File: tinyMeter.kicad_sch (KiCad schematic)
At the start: 93 parts, among them J1 USB_MASTER, J2 DC_POWER, J3 USB_POWER, J4 USBA_OUT_2, J5 USBA_OUT_1, J6 DC_POWER, J7 Debug, J8 External antenna, Q1 100N03A, Q2 100N03A, Q3 100N03A, Q4 SS8050, SW1 SW_Push, SW2 SW_Push, SW3 SW_Push, SW4 SW_Push, SW5 SW_Push, SW6 Boot, SW7 Reset, U1 ESP32-S3, U2 INA219AxD, U3 INA219AxD, U4 INA219AxD, U5 AMS1117-3.3, Y1 Crystal_GND24

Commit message: Working on v2
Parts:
- removed AE1: PCB antenna, Library:ESPRESSIF_ESP32_MIFA_2.4GHz_Right, symbol Device:Antenna_Loop
- removed C1, C2: 10u, Capacitor_SMD:C_0805_2012Metric, symbol Device:C
- removed C10, C11, C16, C17, C19, C20, C21, C22, C23: 100n, Capacitor_SMD:C_0603_1608Metric, symbol Device:C
- removed C12, C15, C18: 1u, Capacitor_SMD:C_0603_1608Metric, symbol Device:C
- removed C13, C14, C3, C6: 10u, Capacitor_SMD:C_0603_1608Metric, symbol Device:C
- removed C4, C5: 10p, Capacitor_SMD:C_0603_1608Metric, symbol Device:C
- removed C7, C8, C9: LNA, Capacitor_SMD:C_0603_1608Metric, symbol Device:C
- removed D1: WS2812B, LED_SMD:LED_WS2812B_PLCC4_5.0x5.0mm_P3.2mm, symbol LED:WS2812B
- removed D2: PWR_LED, LED_SMD:LED_0603_1608Metric, symbol PCM_SL_Devices:LED
- removed DS1: ST77xx, Library:ST77XX, symbol Library:ST77xx
- removed J2: DC_POWER, Connector_BarrelJack:BarrelJack_Horizontal, symbol Connector:Barrel_Jack_MountingPin
- removed J3: USB_POWER, Connector_USB:USB_C_Receptacle_HRO_TYPE-C-31-M-12, symbol Connector:USB_C_Receptacle_USB2.0_16P
- removed J4: USBA_OUT_2, Connector_USB:USB_A_Receptacle_GCT_USB1046, symbol Connector:USB_A
- removed J5: USBA_OUT_1, Connector_USB:USB_A_Receptacle_GCT_USB1046, symbol Connector:USB_A
- removed J7: Debug, Connector_PinSocket_2.54mm:PinSocket_1x04_P2.54mm_Horizontal, symbol Connector_Generic:Conn_01x04
- removed J8: External antenna, Connector_Coaxial:U.FL_Hirose_U.FL-R-SMT-1_Vertical, symbol Connector:Conn_Coaxial
- removed L1, L2: L, Inductor_SMD:L_0603_1608Metric, symbol Device:L
- removed L3: 2n, Inductor_SMD:L_0603_1608Metric, symbol Device:L
- removed Q1, Q2, Q3: 100N03A, Package_TO_SOT_SMD:TO-252-2, symbol Transistor_FET:BUK9832-55A
- removed Q4: SS8050, Package_TO_SOT_SMD:SOT-23, symbol Transistor_BJT:SS8050
- removed R1, R2, R3, R4: 5k1, Resistor_SMD:R_0603_1608Metric, symbol Device:R
- removed R10, R6, R7, R9: 0R, Resistor_SMD:R_0603_1608Metric, symbol Device:R
- removed R11, R5, R8: R025, Resistor_SMD:R_2512_6332Metric, symbol Device:R
- removed R12, R13: 220, Resistor_SMD:R_0603_1608Metric, symbol Device:R
- removed R14, R15, R16, R17, R18, R19, R22, R24, R25, R28, R32, R33, R34: 10k, Resistor_SMD:R_0603_1608Metric, symbol Device:R
- removed R20, R21, R23, R31: 1k, Resistor_SMD:R_0603_1608Metric, symbol Device:R
- removed R26, R27: 2k7, Resistor_SMD:R_0603_1608Metric, symbol Device:R
- removed R29: 60, Resistor_SMD:R_0603_1608Metric, symbol Device:R
- removed R30: 100, Resistor_SMD:R_0603_1608Metric, symbol Device:R
- removed SW6: Boot, Button_Switch_SMD:SW_SPST_B3U-1000P, symbol Switch:SW_Push
- removed SW7: Reset, Button_Switch_SMD:SW_SPST_B3U-1000P, symbol Switch:SW_Push
- removed U1: ESP32-S3, Package_DFN_QFN:QFN-56-1EP_7x7mm_P0.4mm_EP4x4mm, symbol MCU_Espressif:ESP32-S3
- removed U2, U3, U4: INA219AxD, Package_SO:SOIC-8_3.9x4.9mm_P1.27mm, symbol Sensor_Energy:INA219AxD
- removed U5: AMS1117-3.3, Package_TO_SOT_SMD:SOT-223-3_TabPin2, symbol Regulator_Linear:AMS1117-3.3
- removed Y1: Crystal_GND24, Library:OSC_XRCGB40M000F4M00R0, symbol Device:Crystal_GND24
- added C1, C2, C7: 10u, Capacitor_SMD:C_0603_1608Metric, symbol TheEvilRoot:C_0603
- added C3: 1u, Capacitor_SMD:C_0603_1608Metric, symbol TheEvilRoot:C_0603
- added C4, C5, C6: 100n, Capacitor_SMD:C_0603_1608Metric, symbol TheEvilRoot:C_0603
- added J10, J2: USB_IN, TheEvilRoot:USB_C_Receptacle_HRO_TYPE-C-31-M-12, symbol TheEvilRoot:USB_C_Receptacle_USB2.0_16P
- added J11: Debug, Connector_PinHeader_1.27mm:PinHeader_1x06_P1.27mm_Vertical, symbol Connector_Generic:Conn_01x06
- added J3: USB_OUT, TheEvilRoot:USB_C_Receptacle_HRO_TYPE-C-31-M-12, symbol TheEvilRoot:USB_C_Receptacle_USB2.0_16P
- added J4: OLED, Connector_PinSocket_2.54mm:PinSocket_1x04_P2.54mm_Vertical, symbol Connector_Generic:Conn_01x04
- added J5: DC_IN, Connector_BarrelJack:BarrelJack_Horizontal, symbol Connector:Barrel_Jack_MountingPin
- added J7, J8: Conn_01x02, TheEvilRoot:SolderWire-SMD-2pin-2.54mm-D3.0, symbol Connector_Generic:Conn_01x02
- added J9: USB_OUT, TheEvilRoot:TE_292303-1, symbol TheEvilRoot:USB_A_TE_292303-1
- added R1, R4, R5: R100, Resistor_SMD:R_2512_6332Metric, symbol TheEvilRoot:R_2512
- added R10, R11, R12, R13, R6, R7, R8, R9: 10k, Resistor_SMD:R_0603_1608Metric, symbol TheEvilRoot:R_0603
- added R14, R15, R2, R3: 5k1, Resistor_SMD:R_0603_1608Metric, symbol TheEvilRoot:R_0603
- added R16, R17, R18, R19, R20: R, Resistor_SMD:R_0603_1608Metric, symbol TheEvilRoot:R_0603
- added R21, R22: 2k7, Resistor_SMD:R_0603_1608Metric, symbol TheEvilRoot:R_0603
- added U1: AP2112K-3.3, Package_TO_SOT_SMD:SOT-23-5, symbol Regulator_Linear:AP2112K-3.3
- added U2: INA3221AIRGVR, TheEvilRoot:QFN65P400X400X100-17N, symbol TheEvilRoot:INA3221AIRGVR
- added U3: ESP32-S3-WROOM-1, TheEvilRoot:ESP32-S3-WROOM-1, symbol TheEvilRoot:ESP32-S3-WROOM-1
- J1: value USB_MASTER -> USB_C_Receptacle_USB2.0_16P; footprint Connector_USB:USB_C_Receptacle_HRO_TYPE-C-31-M-12 -> TheEvilRoot:USB_C_Receptacle_HRO_TYPE-C-31-M-12; symbol Connector:USB_C_Receptacle_USB2.0_16P -> TheEvilRoot:USB_C_Receptacle_USB2.0_16P
- J6: value DC_POWER -> DC_OUT
- SW1: value SW_Push -> A1; footprint Button_Switch_SMD:SW_SPST_B3U-1000P -> TheEvilRoot:IT-1185AP
- SW2: value SW_Push -> A2; footprint Button_Switch_SMD:SW_SPST_B3U-1000P -> TheEvilRoot:IT-1185AP
- SW3: value SW_Push -> A3; footprint Button_Switch_SMD:SW_SPST_B3U-1000P -> TheEvilRoot:IT-1185AP
- SW4: value SW_Push -> A4; footprint Button_Switch_SMD:SW_SPST_B3U-1000P -> TheEvilRoot:IT-1185AP
- SW5: value SW_Push -> A0; footprint Button_Switch_SMD:SW_SPST_B3U-1000P -> TheEvilRoot:IT-1185AP
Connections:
- net DC_POWER_GND is gone; now on net GND: J6.2
- net KEYPAD_K1 is gone; now on net +3V3: SW1.1
- net KEYPAD_K2 is gone; now on net +3V3: SW2.1
- net KEYPAD_K3 is gone; now on net +3V3: SW3.1
- net KEYPAD_K4 is gone; now on net +3V3: SW4.1
- net KEYPAD_K5 is gone; now on net +3V3: SW5.1
- net +3V3: now also C2.1, C3.1, C4.1, C5.1, C6.1, J11.1 (Pin_1), J4.2 (Pin_2), R10.1, R11.1, R12.1, R13.1, R21.1, R22.1, R6.1, R7.1, R8.1, R9.1, U1.5 (VOUT), U2.16 (VPU), U2.4 (VS), U3.2 (3V3)
- net ESP_EN: now also C7.1, J11.4 (Pin_4), R13.2, U3.3 (EN)
- net ESP_RX: now also J11.3 (Pin_3), U3.36 (RXD0)
- net ESP_TX: now also J11.2 (Pin_2), U3.37 (TXD0)
- net GND: now also C1.2, C2.2, C3.2, C4.2, C5.2, C6.2, C7.2, J10.A1 (GND), J10.A12 (GND), J10.B1 (GND), J10.B12 (GND), J11.6 (Pin_6), J2.A1 (GND), J2.A12 (GND), J2.B1 (GND), J2.B12 (GND), J3.A1 (GND), J3.A12 (GND), J3.B1 (GND), J3.B12 (GND), J4.1 (Pin_1), J5.2, J7.1 (Pin_1), J8.1 (Pin_1), J9.4 (GND), R14.2, R15.2, R2.2, R3.2, U1.2 (GND), U2.17 (EXP), U2.3 (GND), U2.5 (A0), U3.1 (GND), U3.40 (GND), U3.41 (GND)
- net METER_SCL: now also R10.2, U2.6 (SCL), U3.35 (IO42)
- net METER_SDA: now also R11.2, U2.7 (SDA), U3.34 (IO41)
- net USB_MASTER_CC1: now also R3.1
- net USB_MASTER_CC2: now also R2.1
- net USB_MASTER_D+: now also U3.14 (USB_D+)
- net USB_MASTER_D-: now also U3.13 (USB_D-)
- net at SW2.2: now also R17.1
- net at SW3.2: now also R18.1
- net at SW4.2: now also R19.1
- net at SW1.2: now also R16.1
- net at SW5.2: now also R20.1
- net DC_POWER_VCC renamed METER_3-
- net METER_3-: now also R4.2, U2.1 (IN-3)
- net USB_VBUS renamed VBUS
- net VBUS: now also C1.1, U1.1 (VIN), U1.3 (EN)
- new net ESP_BOOT: J11.5 (Pin_5), R12.2, U3.27 (IO0)
- new net METER_1+: J2.A4 (VBUS), J2.A9 (VBUS), J2.B4 (VBUS), J2.B9 (VBUS), J7.2 (Pin_2), R1.1, U2.12 (IN+1)
- new net METER_1-: J3.A4 (VBUS), J3.A9 (VBUS), J3.B4 (VBUS), J3.B9 (VBUS), J8.2 (Pin_2), R1.2, U2.11 (IN-1)
- new net METER_2+: J10.A4 (VBUS), J10.A9 (VBUS), J10.B4 (VBUS), J10.B9 (VBUS), R5.1, U2.15 (IN+2)
- new net METER_2-: J9.1 (VBUS), R5.2, U2.14 (IN-2)
- new net METER_3+: J5.1, R4.1, U2.2 (IN+3)
- new net METER_CRIT: R6.2, U2.9 (CRITICAL), U3.32 (IO39)
- new net METER_TIMING: R8.2, U2.13 (TC), U3.26 (IO45)
- new net METER_VALID: R7.2, U2.10 (PV), U3.31 (IO38)
- new net METER_WARN: R9.2, U2.8 (WARNING), U3.33 (IO40)
- new net OLED_SCL: J4.3 (Pin_3), R22.2, U3.19 (IO11)
- new net OLED_SDA: J4.4 (Pin_4), R21.2, U3.18 (IO10)
- new net SW_A0: R20.2, U3.12 (IO8)
- new net SW_A1: R16.2, U3.11 (IO18)
- new net SW_A2: R17.2, U3.10 (IO17)
- new net SW_A3: R18.2, U3.9 (IO16)
- new net SW_A4: R19.2, U3.8 (IO15)
- new net USB_A_CC1: J10.A5 (CC1), R14.1
- new net USB_A_CC2: J10.B5 (CC2), R15.1
- new net USB_A_D+: J10.A6 (D+), J10.B6 (D+), J9.3 (D+)
- new net USB_A_D-: J10.A7 (D-), J10.B7 (D-), J9.2 (D-)
- new net USB_C_CC1: J2.A5 (CC1), J3.A5 (CC1)
- new net USB_C_CC2: J2.B5 (CC2), J3.B5 (CC2)
- new net USB_C_D1+: J2.B6 (D+), J3.B6 (D+)
- new net USB_C_D1-: J2.A7 (D-), J3.A7 (D-)
- new net USB_C_D2+: J2.A6 (D+), J3.A6 (D+)
- new net USB_C_D2-: J2.B7 (D-), J3.B7 (D-)
- new net USB_C_SBU1: J2.A8 (SBU1), J3.A8 (SBU1)
- new net USB_C_SBU2: J2.B8 (SBU2), J3.B8 (SBU2)
- no-connect marks 39 -> 28
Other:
- note added: "TODO: 1. Test points for - Meter +/- - 3.3V - Meter open-drains params 2. Debug LEDs for MCU 3. LEDs for open-drains meter outputs"

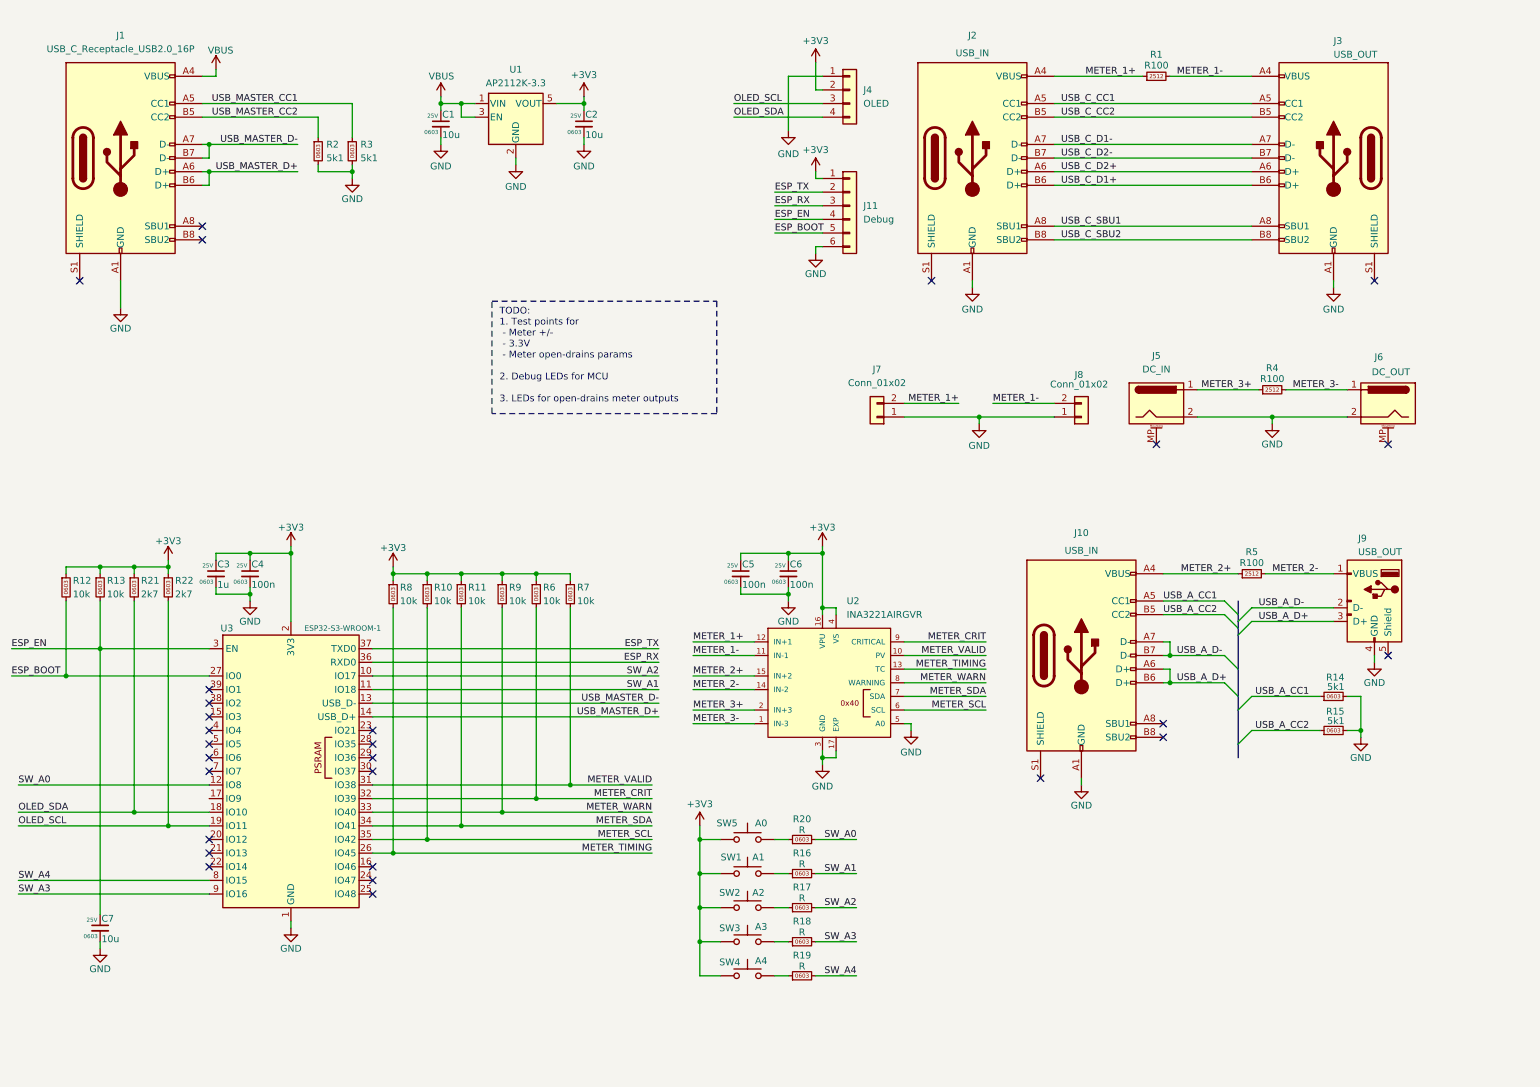
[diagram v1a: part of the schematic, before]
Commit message: Version 2 finish
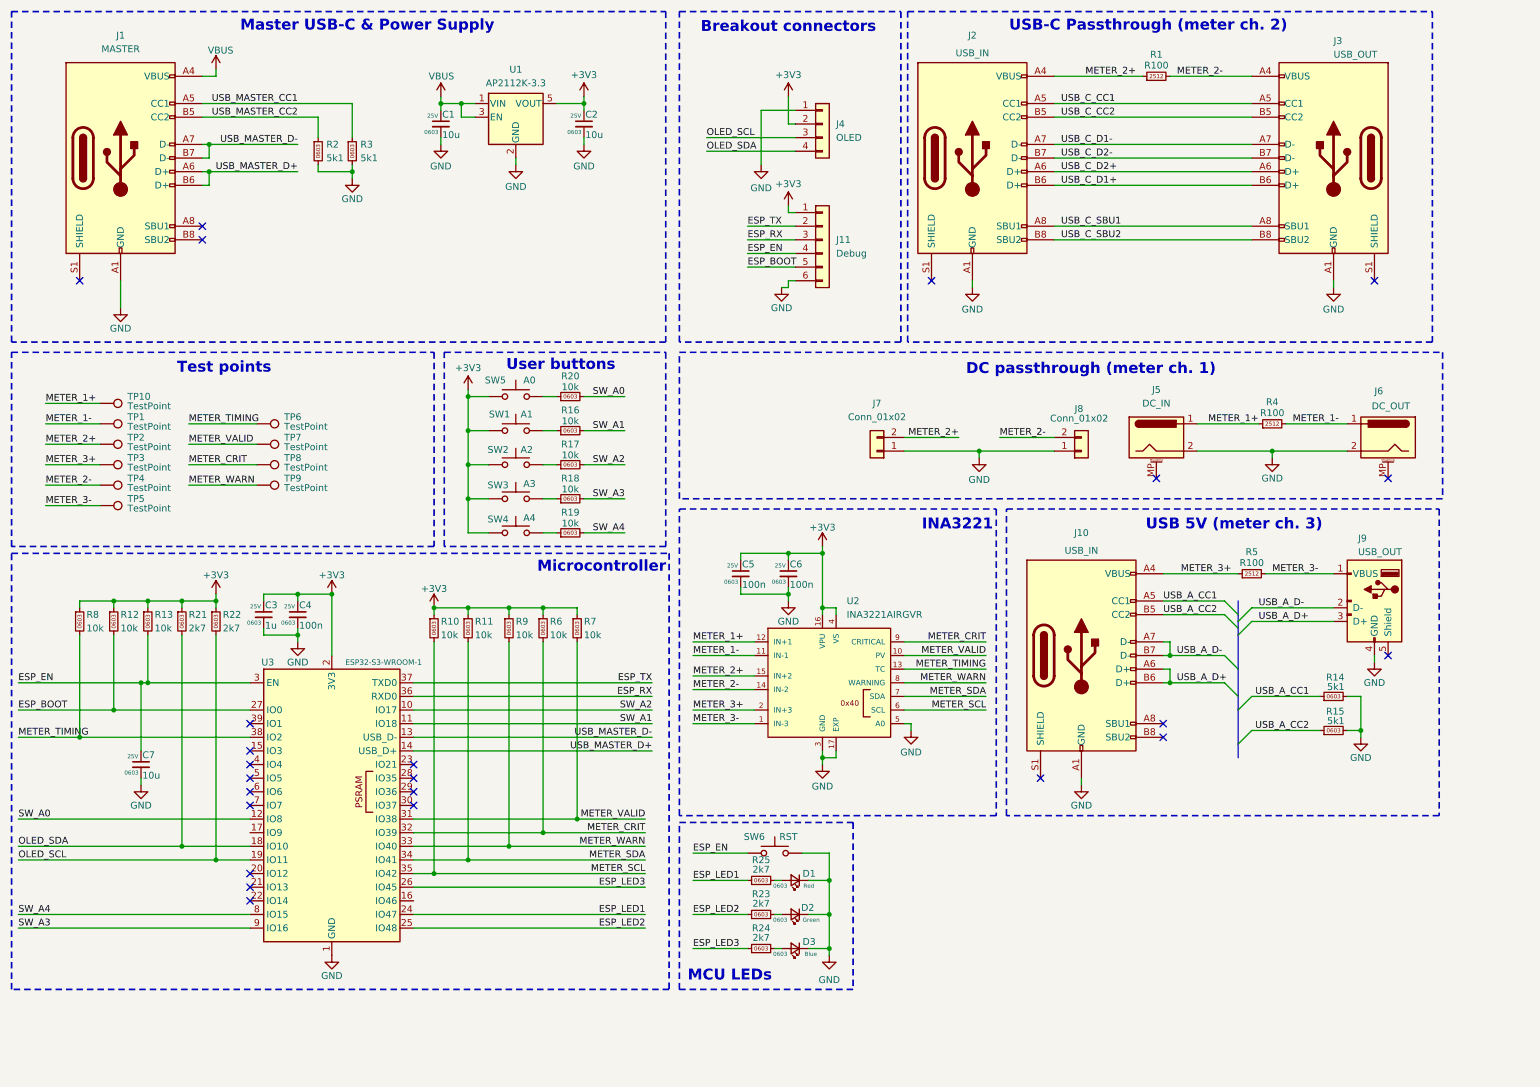
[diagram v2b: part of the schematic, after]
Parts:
- added D1: Red, LED_SMD:LED_0603_1608Metric, symbol TheEvilRoot:LED_0603_Red
- added D2: Green, LED_SMD:LED_0603_1608Metric, symbol TheEvilRoot:LED_0603_Green
- added D3: Blue, LED_SMD:LED_0603_1608Metric, symbol TheEvilRoot:LED_0603_Blue
- added R23, R24, R25: 2k7, Resistor_SMD:R_0603_1608Metric, symbol TheEvilRoot:R_0603
- added SW6: RST, TheEvilRoot:KLS7-TS3401, symbol Switch:SW_Push
- added TP1, TP10, TP2, TP3, TP4, TP5, TP6, TP7, TP8, TP9: TestPoint, TestPoint:TestPoint_Pad_D1.0mm, symbol Connector:TestPoint
- J1: value USB_C_Receptacle_USB2.0_16P -> MASTER
- J7, J8: footprint TheEvilRoot:SolderWire-SMD-2pin-2.54mm-D3.0 -> Connector_PinHeader_2.54mm:PinHeader_1x02_P2.54mm_Vertical
- R16, R17, R18, R19, R20: value R -> 10k
- SW1, SW2, SW3, SW4, SW5: footprint TheEvilRoot:IT-1185AP -> TheEvilRoot:KLS7-TS3401
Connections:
- net ESP_EN: now also SW6.1
- net GND: now also D1.1 (K), D2.1 (K), D3.1 (K), SW6.2
- net METER_1+: now also J5.1, R4.1, TP10.1; no longer J2.A4 (VBUS), J2.A9 (VBUS), J2.B4 (VBUS), J2.B9 (VBUS), J7.2 (Pin_2), R1.1
- net METER_1-: now also J6.1, R4.2, TP1.1; no longer J3.A4 (VBUS), J3.A9 (VBUS), J3.B4 (VBUS), J3.B9 (VBUS), J8.2 (Pin_2), R1.2
- net METER_2+: now also J2.A4 (VBUS), J2.A9 (VBUS), J2.B4 (VBUS), J2.B9 (VBUS), J7.2 (Pin_2), R1.1, TP2.1; no longer J10.A4 (VBUS), J10.A9 (VBUS), J10.B4 (VBUS), J10.B9 (VBUS), R5.1
- net METER_2-: now also J3.A4 (VBUS), J3.A9 (VBUS), J3.B4 (VBUS), J3.B9 (VBUS), J8.2 (Pin_2), R1.2, TP4.1; no longer J9.1 (VBUS), R5.2
- net METER_3+: now also J10.A4 (VBUS), J10.A9 (VBUS), J10.B4 (VBUS), J10.B9 (VBUS), R5.1, TP3.1; no longer J5.1, R4.1
- net METER_3-: now also J9.1 (VBUS), R5.2, TP5.1; no longer J6.1, R4.2
- net METER_CRIT: now also TP8.1
- net METER_TIMING: now also U3.38 (IO2), TP6.1; no longer U3.26 (IO45)
- net METER_VALID: now also TP7.1
- net METER_WARN: now also TP9.1
- net ESP_LED1: now reaches U3.24 (IO47)
- net ESP_LED1: now also R25.1
- net ESP_LED2: now reaches U3.25 (IO48)
- net ESP_LED2: now also R23.1
- new net: D1.2 (A), R25.2
- new net: D2.2 (A), R23.2
- new net: D3.2 (A), R24.2
- new net ESP_LED3: R24.1, U3.26 (IO45)
- no-connect marks 28 -> 24
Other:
- note added: "Breakout connectors"
- note added: "DC passthrough (meter ch. 1)"
- note added: "INA3221"
- note added: "MCU LEDs"
- note added: "Master USB-C & Power Supply"
- note added: "Microcontroller"
- note added: "Test points"
- note added: "USB 5V (meter ch. 3)"
- note added: "USB-C Passthrough (meter ch. 2)"
- note added: "User buttons"
- note removed: "TODO: 1. Test points for - Meter +/- - 3.3V - Meter open-drains params 2. Debug LEDs for MCU 3. LEDs for open-drains meter outputs"
- company: (none) -> TheEvilRoot
- title: (none) -> tinyMeter
- moved on the sheet: C3, C4, C7, J11, J4, J5, J6, J7, J8, R10, R11, R12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

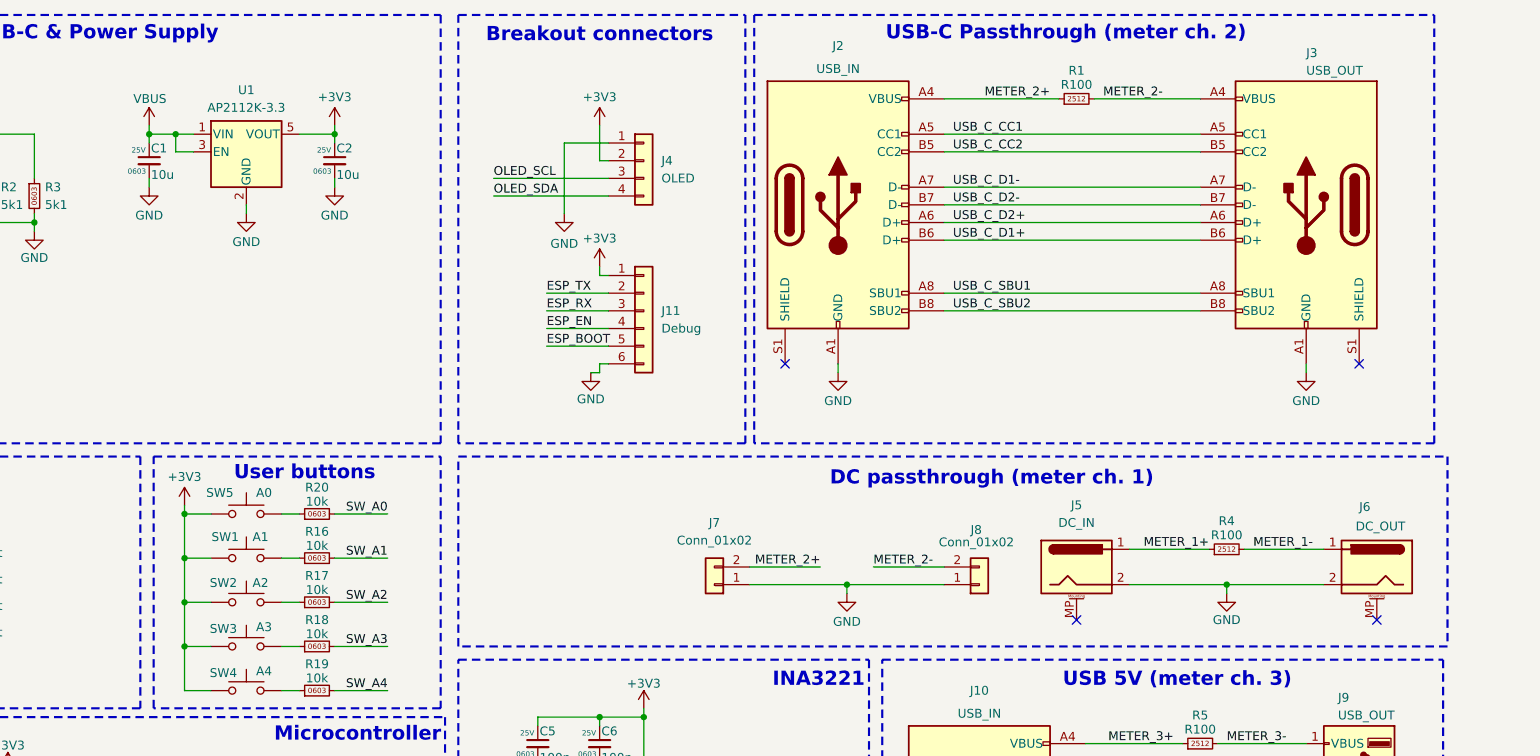
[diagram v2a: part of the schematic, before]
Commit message: Working
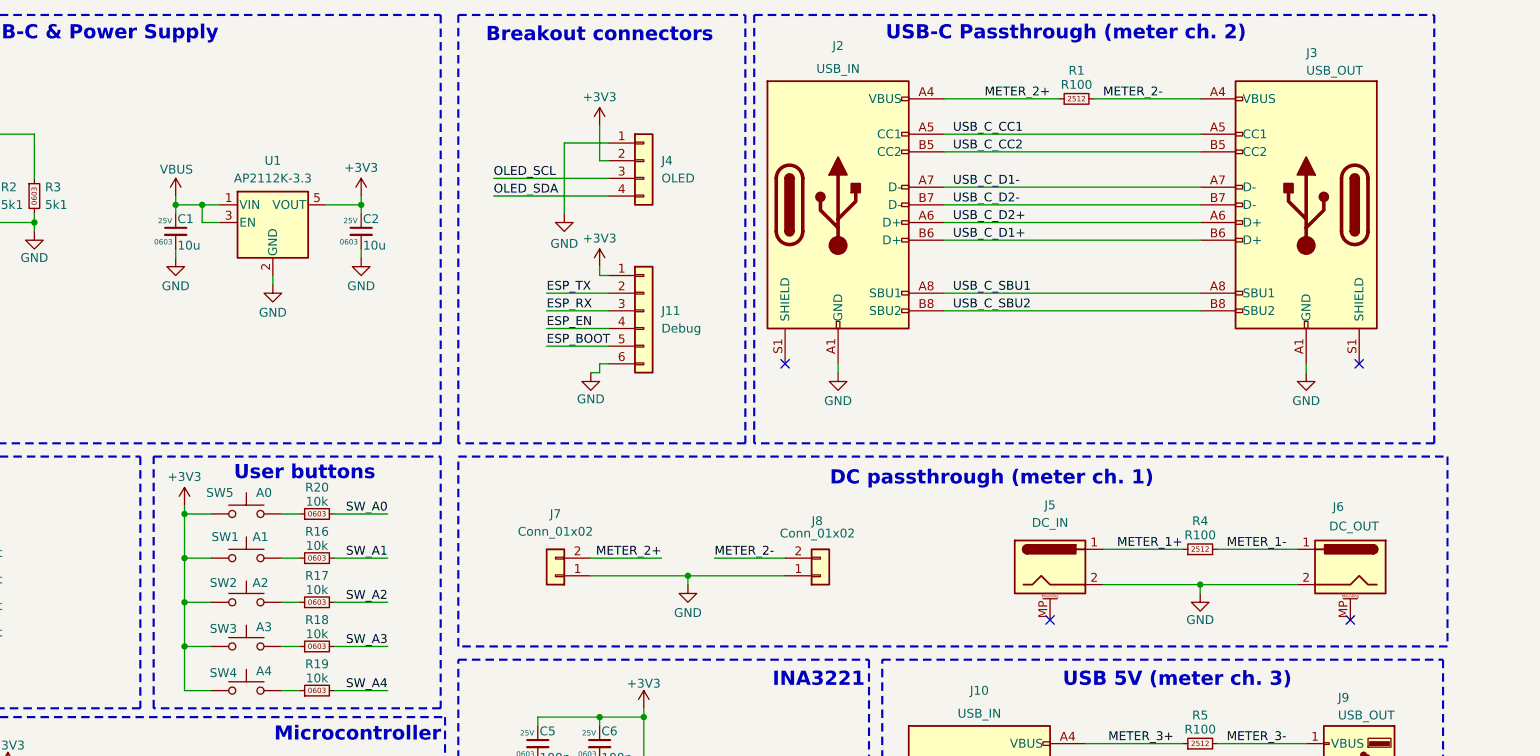
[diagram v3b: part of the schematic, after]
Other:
- moved on the sheet: C1, C2, J5, J6, J7, J8, R4, U1
